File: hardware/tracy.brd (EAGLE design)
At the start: 58.5 x 38 mm, 77 parts, among them IC1 SIM900, J1 U.FL, J2 U.FL, Q4 si2305cd, T2 BC846, U1 SPX5205 3v3, U2 3339, U3 TC1014 2V8, Y1 32768Hz CFPX-217 12.5pF

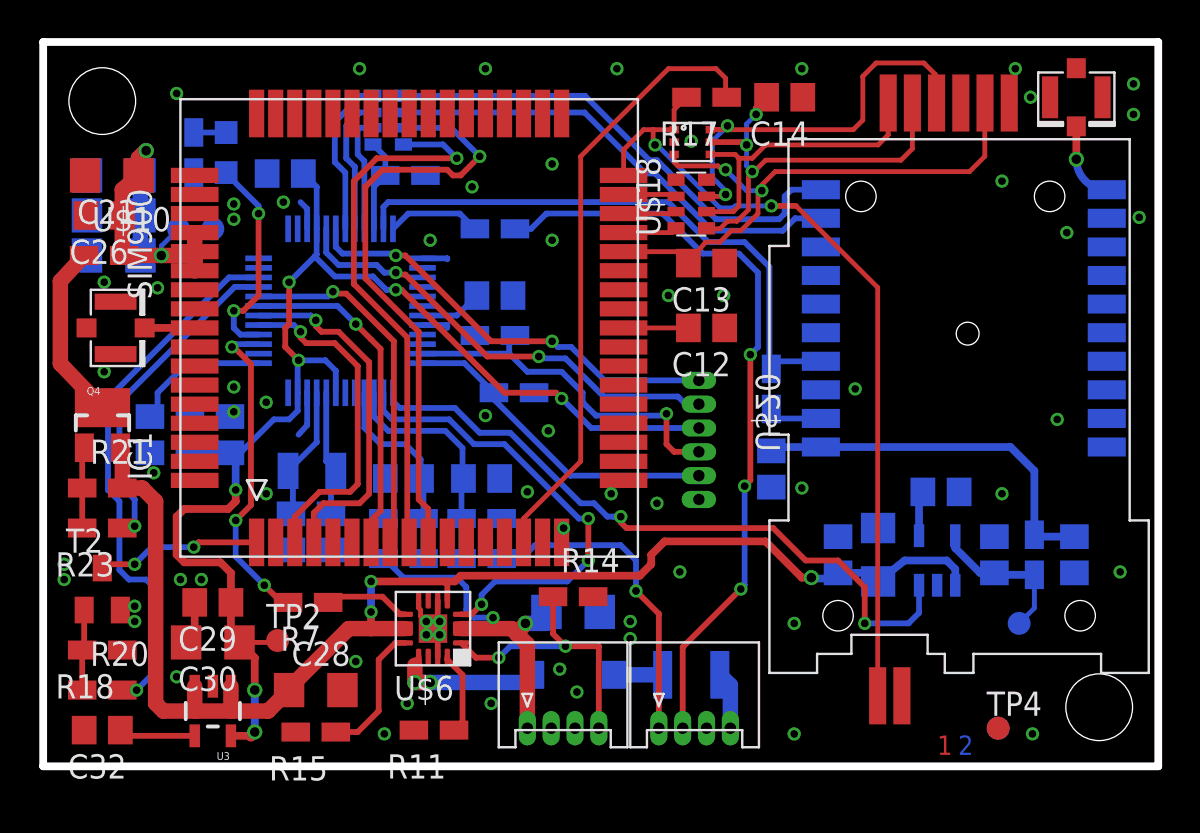
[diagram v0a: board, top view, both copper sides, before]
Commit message: checks
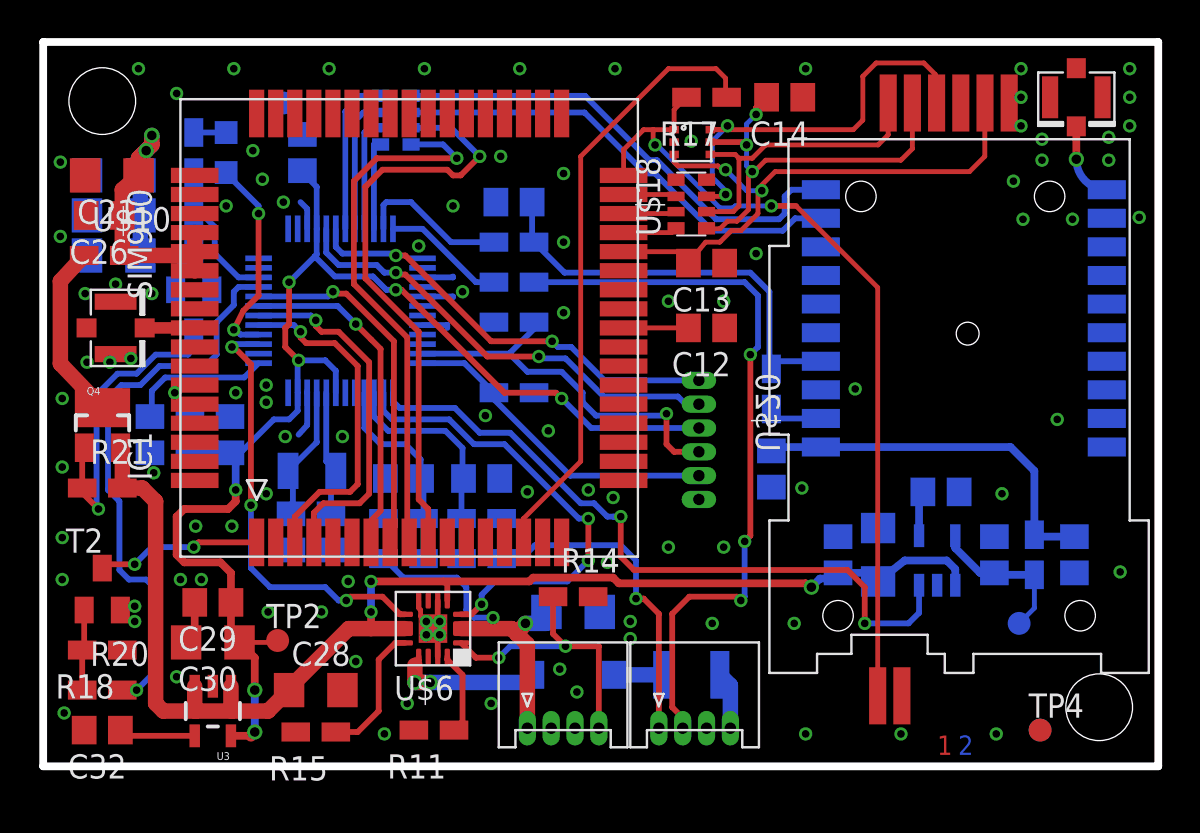
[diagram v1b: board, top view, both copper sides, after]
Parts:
- removed R2: 2k2, rcl:R0805W
- removed R7: 470, rcl:R0805W
- removed TP1: TPTP12R, testpad:TP12R
- added R8: 330, rcl:R0805W
- added T1: BC846, transistor:SOT23
- C11: value 220nF -> 10uF
- C18: value NA 100nF -> DNP 100nF
- R21: value 100k -> 10k
- R24: value 240k -> 240K
- R4: value 240k -> 1M3
- R5: value 4k7 -> 1k
- moved R23 16.3 mm to (7.90, 28.1), flipped to the bottom, turned to 270 degrees
- moved TP5 7.57 mm to (12.6, 34.8)
- moved C11 5.00 mm to (24.7, 29.6), turned to 0 degrees
- moved R5 2.97 mm to (24.7, 25.4)
- moved TP4 2.20 mm to (52.3, 1.90)
- moved TP6 2.20 mm to (52.3, 1.90)
- moved C9 1.42 mm to (13.6, 32.2), turned to 270 degrees
- moved R35 1.22 mm to (24.7, 23.3)
- moved U$2 0.40 mm to (18.5, 33.9)
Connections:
- removed net 41: U$1.41
- removed net N$5: R2.2, U$1.34, U$2.1
- removed net VBACKUP: R1.2, U$1.35, U2.4
- new net 43: U$1.43
- new net GPS_BKP: R8.2, U$1.35
- new net N$11: C11.1, R1.2, R8.1, U2.4
- net CH: now also U$6.9; no longer R7.2
- net GND: now also T1.2, U$1.39, U$1.41; no longer R2.1
- net GPRS_EN: now also U$1.22; no longer U$1.21
- net GPRS_POW: now also U$1.21; no longer U$1.22
- net N$10: now also U$1.34, U$2.1; no longer R7.1, U$6.9
- net N$48: now also T1.3; no longer R23.2
- net N$7: now also R23.2, T1.1; no longer C11.1, U$1.43
- net VBAT: no longer TP1.TP
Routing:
- net VBACKUP: track 30.9 -> 0.00 mm
- net N$11: track 0.00 -> 22.6 mm
- net N$48: track 4.23 -> 16.6 mm, vias 0 -> 1
- net GPRS_EN: track 17.3 -> 5.74 mm, vias 1 -> 0
- net GPS_BKP: track 0.00 -> 7.98 mm
- net CH: track 17.0 -> 22.8 mm
- net N$5: track 4.94 -> 0.00 mm
- net GND: track 14.8 -> 16.7 mm, vias 64 -> 98
- net PW_EN: track 4.96 -> 6.46 mm
- net VIN: track 70.4 -> 68.9 mm
- net N$12: track 39.9 -> 38.7 mm
- net GPRS_POW: track 28.6 -> 29.8 mm
- net TEST: track 19.0 -> 20.1 mm
- net 3V3_EN: track 36.2 -> 37.3 mm
- net N$7: track 3.28 -> 2.44 mm
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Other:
- board text added: "Petre Rodan 201405 rev1"
- board text removed: "Vbat"
- board text removed: "peter 201401 rev1"
